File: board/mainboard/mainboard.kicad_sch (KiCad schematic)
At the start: 39 parts, among them J1 QWIIC, J2 QWIIC, J3 UPDI, U1 ATMEGA808, U2 Si4463, U3 BME280, U4 MAX-M8C, U5 TPS613221A, Y1 30MHz

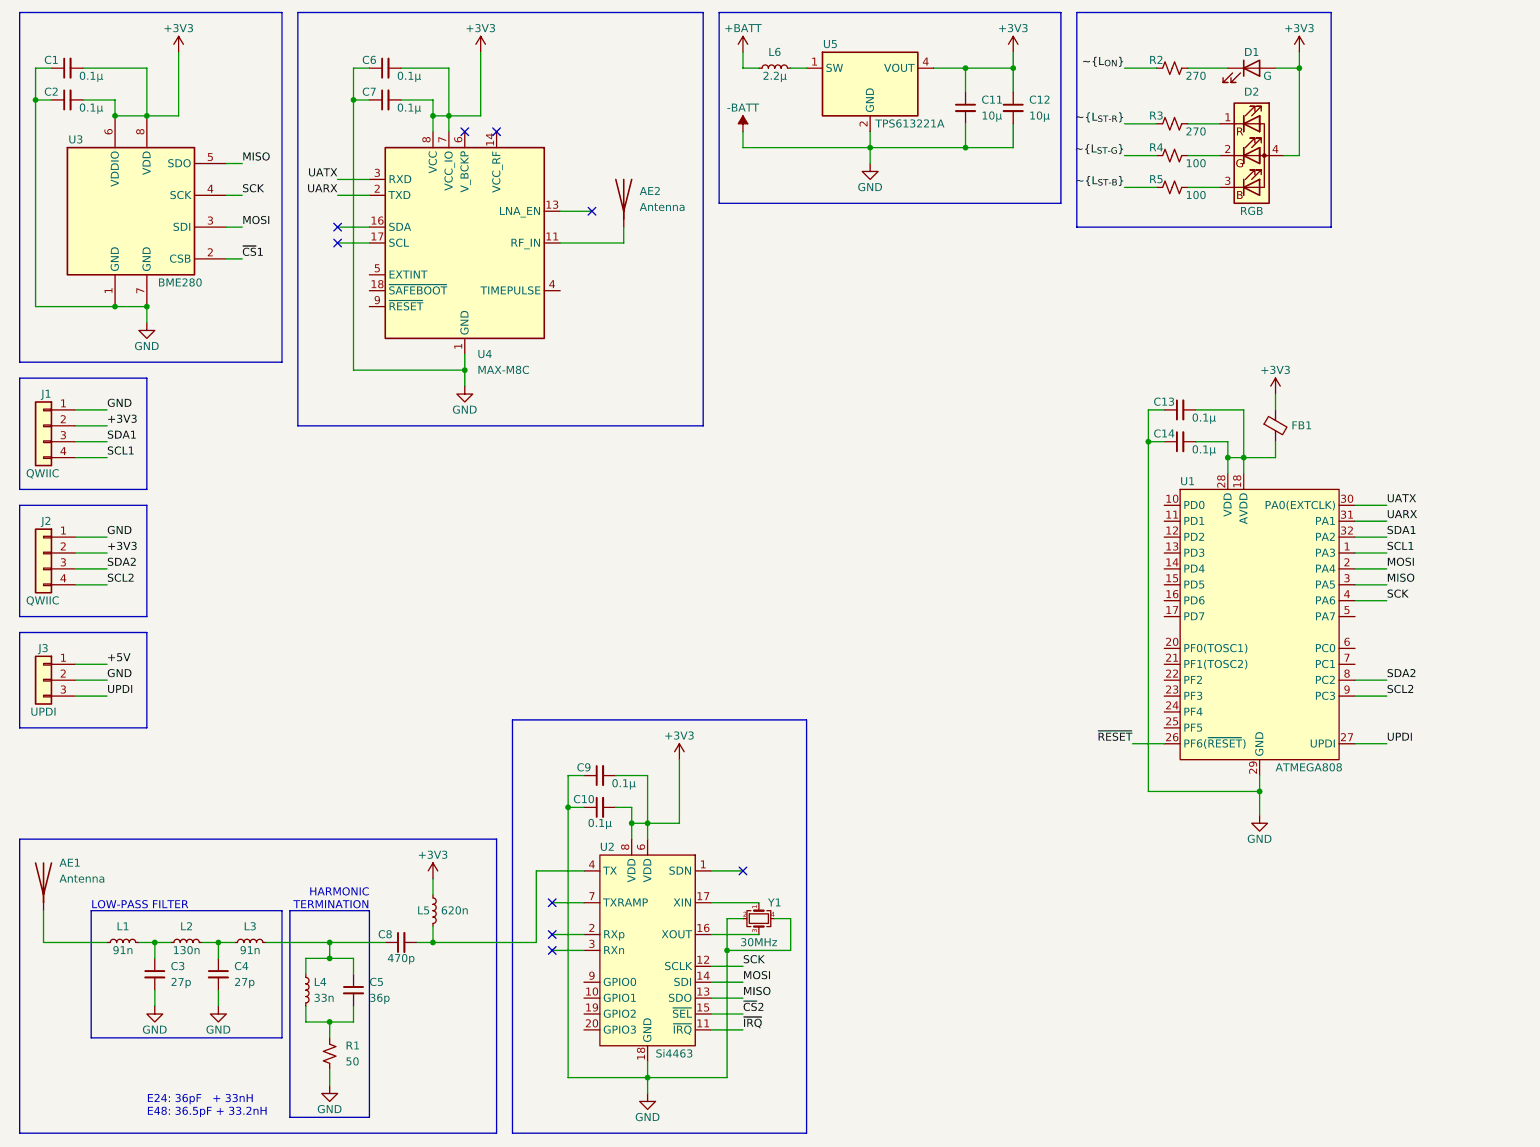
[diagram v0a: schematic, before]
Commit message: latest PCB design update (will commit better henceforth)
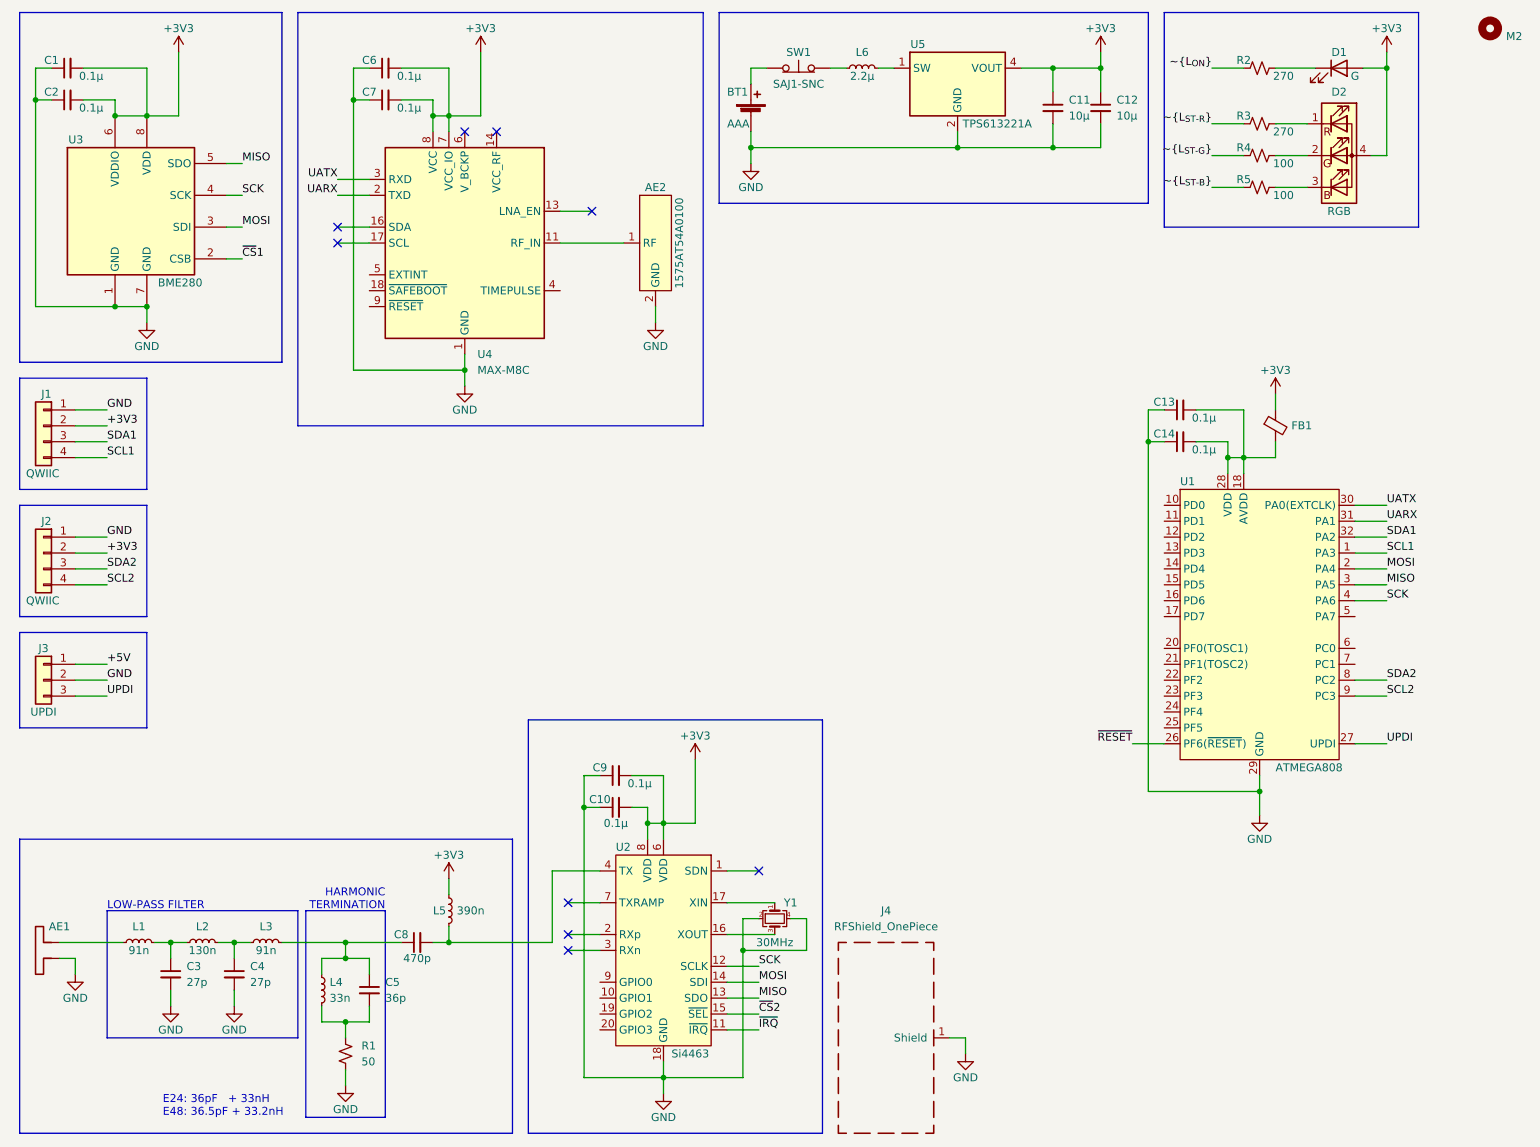
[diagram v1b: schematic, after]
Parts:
- removed AE1, AE2: Antenna, symbol Device:Antenna
- added AE1: Antenna_Dipole, Dipole:AE_Pad, symbol Device:Antenna_Dipole
- added AE2: 1575AT54A0100, 1575AT54:Johanson_AT54, symbol 1575AT54:1575AT54A0100
- added BT1: AAA, Battery:BatteryHolder_Keystone_2466_1xAAA, symbol Device:Battery_Cell
- added H1: M2, MountingHole:MountingHole_2.2mm_M2, symbol Mechanical:MountingHole
- added J4: RFShield_OnePiece, RF_Shielding:Wuerth_36103205_20x20mm, symbol Device:RFShield_OnePiece
- added SW1: SAJ1-SNC, SAJ13:SAJ1______N88SNCPT_, symbol Switch:SW_Push_Open
- C1, C10, C13, C14, C2, C6, C7, C9: footprint Capacitor_SMD:C_0603_1608Metric_Pad1.08x0.95mm_HandSolder -> Capacitor_SMD:C_0402_1005Metric
- C11, C12: footprint Capacitor_SMD:C_0805_2012Metric_Pad1.18x1.45mm_HandSolder -> Capacitor_SMD:C_0603_1608Metric
- C3, C4, C5, C8: footprint Capacitor_SMD:C_0603_1608Metric_Pad1.08x0.95mm_HandSolder -> Capacitor_SMD:C_0603_1608Metric
- D1: footprint LED_SMD:LED_0603_1608Metric_Pad1.05x0.95mm_HandSolder -> LED_SMD:LED_0603_1608Metric
- FB1: footprint Inductor_SMD:L_0805_2012Metric_Pad1.05x1.20mm_HandSolder -> Inductor_SMD:L_0805_2012Metric
- J3: footprint Connector_PinHeader_2.54mm:PinHeader_1x03_P2.54mm_Vertical -> Connector_PinHeader_2.54mm:PinHeader_1x03_P2.54mm_Horizontal
- L1, L2, L3, L4: footprint Inductor_SMD:L_0603_1608Metric_Pad1.05x0.95mm_HandSolder -> Inductor_SMD:L_0603_1608Metric
- L5: value 620n -> 390n; footprint Inductor_SMD:L_1008_2520Metric_Pad1.43x2.20mm_HandSolder -> Inductor_SMD:L_0603_1608Metric
- R1, R2, R3, R4, R5: footprint Resistor_SMD:R_0603_1608Metric_Pad0.98x0.95mm_HandSolder -> Resistor_SMD:R_0603_1608Metric
- Y1: footprint (none) -> Crystal:Crystal_SMD_3225-4Pin_3.2x2.5mm
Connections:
- net at L1.1: now also AE1.2
- net at U4.11 (RF_IN): now also AE2.1 (RF)
- net +BATT: no longer names the net of L6.1
- net +BATT: now also SW1.1 (A)
- net -BATT renamed GND
- net GND: now also AE1.1, AE2.2 (GND), AE2.4 (GND), BT1.2 (-), J4.1 (Shield)
- new net: BT1.1 (+), SW1.2 (B)
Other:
- moved on the sheet: C10, C11, C12, C3, C4, C5, C8, C9, D1, D2, L1, L2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
